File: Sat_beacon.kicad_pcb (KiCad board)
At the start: 4 copper layers, 123.9 x 79.5 mm, 126 parts, among them IC1 LMX2581ESQE_NOPB, IC2 LMX2581ESQE_NOPB, J1 Conn_01x05_Pin, J2 Conn_01x03_Pin, J4 SMA, J5 SMA, J6 Conn_01x04_Pin, Q1 BC817-40, Q2 BC817-40, Q3 BC817-40, Q4 BC817-40, SW1 B1407, SW2 SW_Omron_B3FS, SW3 SW_Omron_B3FS, SW4 SW_Omron_B3FS, SW5 SW_Omron_B3FS, U1 LD1117DT33, U2 LD1117DT33, U3 LD1117DT33, U4 1720BL15B0050002E, U5 1720BL15B0050002E, U7 STM32C031C6Tx, Y1 FT2MHUPM10.0-T1

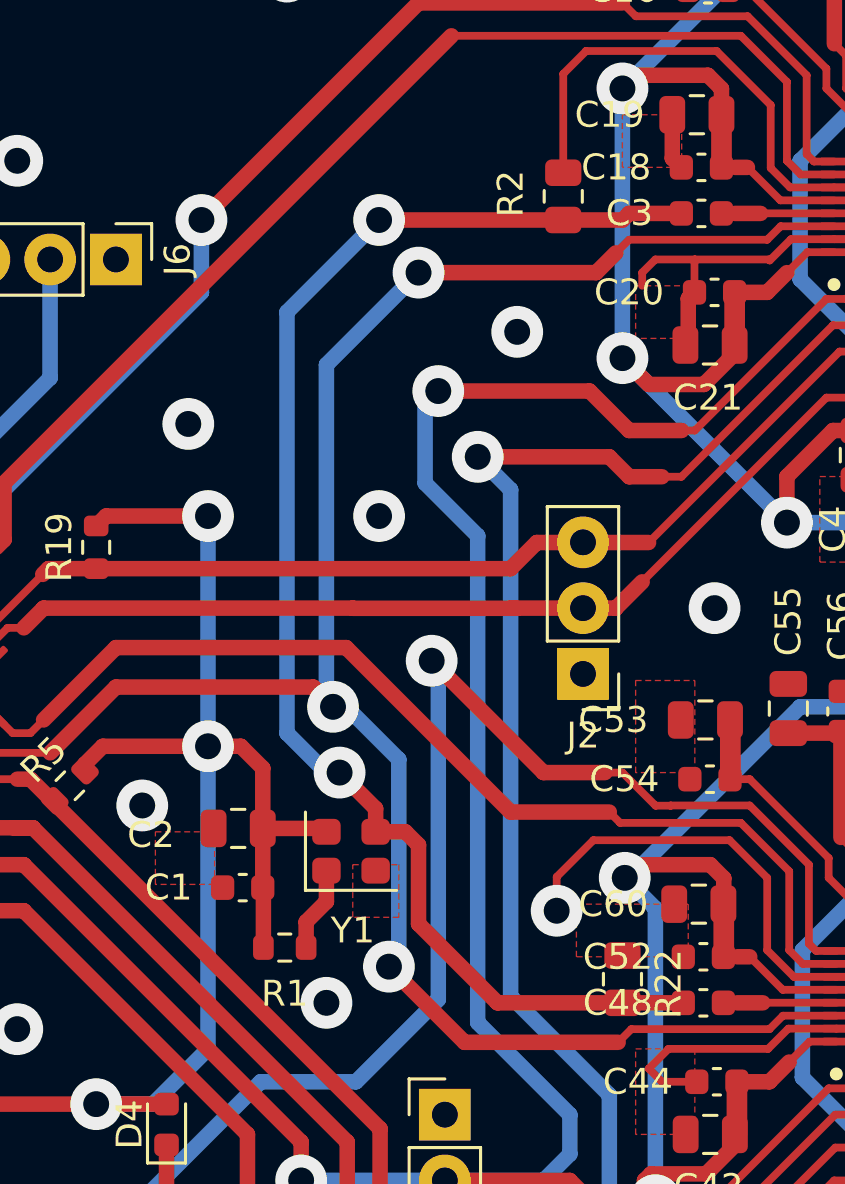
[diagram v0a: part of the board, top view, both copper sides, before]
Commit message: PCB improvements
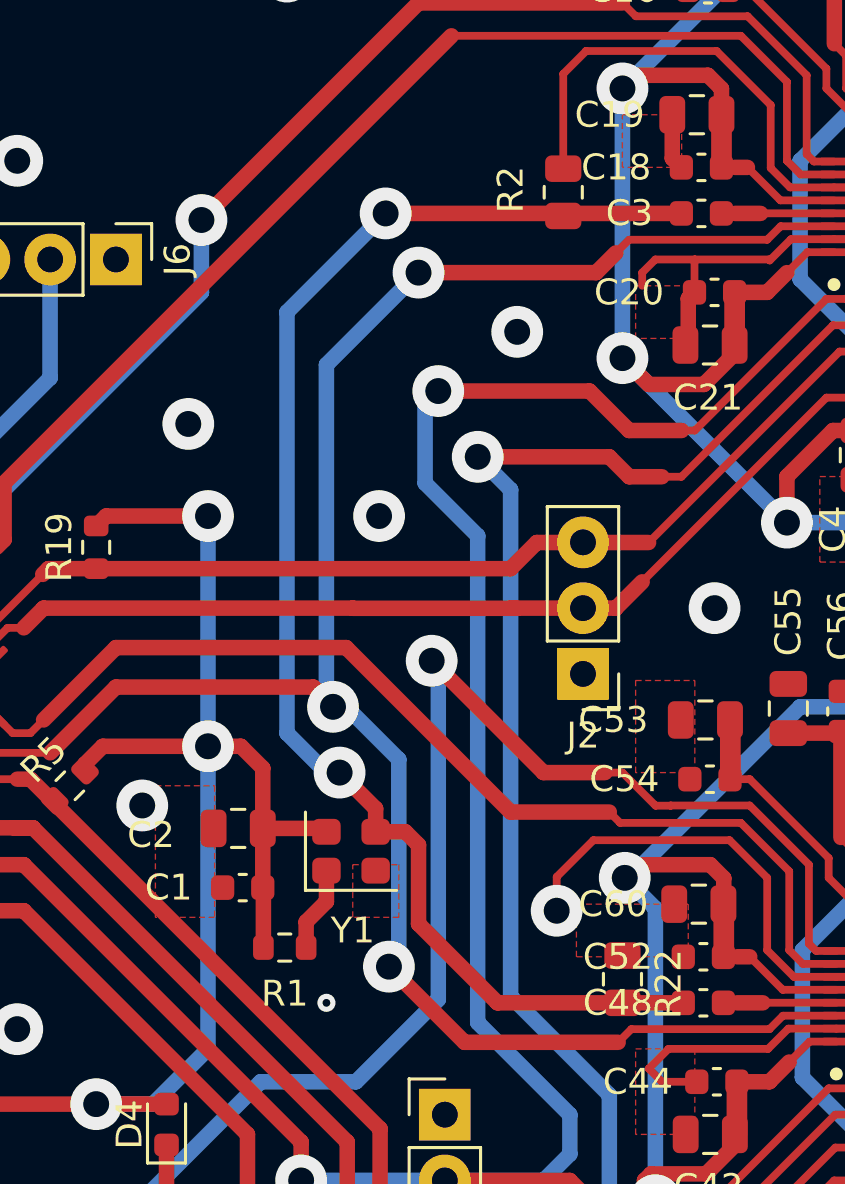
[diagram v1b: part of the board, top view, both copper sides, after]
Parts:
- moved R2 0.16 mm to (133.3, 75.7)
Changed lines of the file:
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@@
 	(footprint "Resistor_SMD:R_0805_2012Metric"
 		(layer "F.Cu")
-		(at 133.297317 75.857676 90)
+		(at 133.297317 75.700677 90)
 		(descr "Resistor SMD 0805 (2012 Metric), square (rectangular) end terminal, IPC-7351 nominal, (Body size source: IPC-SM-782 page 72, https://www.pcb-3d.com/wordpress/wp-content/uploads/ipc-sm-782a_amendment_1_and_2.pdf), generated with kicad-footprint-generator")
 		(tags "resistor")
@@
 	(via
 		(at 124.153317 106.996176)
-		(size 2)
-		(drill 1)
+		(size 0.7)
+		(drill 0.3)
 		(layers "F.Cu" "B.Cu")
 		(free yes)
@@
 	)
 	(segment
-		(start 135.837317 76.516177)
-		(end 135.583317 76.770176)
-		(width 0.6)
-		(layer "F.Cu")
-		(net 4)
-	)
-	(segment
 		(start 127.709317 100.900176)
 		(end 127.201318 100.392177)
@@
 	)
 	(segment
-		(start 135.583317 76.770176)
-		(end 133.297317 76.770176)
-		(width 0.6)
-		(layer "F.Cu")
-		(net 4)
-	)
-	(segment
 		(start 135.925593 106.996176)
 		(end 137.944592 106.996177)
@@
 	)
 	(segment
-		(start 133.297317 76.770176)
-		(end 126.185318 76.770176)
-		(width 0.6)
-		(layer "F.Cu")
-		(net 4)
-	)
-	(segment
 		(start 127.709317 103.948177)
 		(end 127.709317 100.900176)
@@
 	)
 	(segment
-		(start 135.837317 76.516177)
+		(start 126.439317 76.516177)
 		(end 137.856317 76.516177)
 		(width 0.6)
@@
 	)
 	(via
-		(at 126.185318 76.770176)
+		(at 126.439317 76.516177)
 		(size 2)
 		(drill 1)
@@
 	(segment
 		(start 124.153317 98.106177)
-		(end 122.629317 96.582177)
+		(end 124.661317 98.106176)
 		(width 0.6)
 		(layer "B.Cu")
@@
 	(segment
 		(start 122.629317 80.326177)
-		(end 126.185318 76.770176)
+		(end 122.629317 96.582177)
 		(width 0.6)
 		(layer "B.Cu")
@@
 	)
 	(segment
-		(start 122.629317 96.582177)
+		(start 126.439317 76.516177)
 		(end 122.629317 80.326177)
 		(width 0.6)
@@
 	)
 	(segment
-		(start 124.661317 98.106176)
+		(start 122.629317 96.582177)
 		(end 124.153317 98.106177)
 		(width 0.6)
@@
 		(name "$teardrop_padvia$")
 		(hatch none 0.1)
-		(priority 30002)
+		(priority 30003)
 		(attr
 			(teardrop
@@
 		(name "$teardrop_padvia$")
 		(hatch none 0.1)
-		(priority 30001)
+		(priority 30006)
 		(attr
 			(teardrop
@@
 		(name "$teardrop_padvia$")
 		(hatch none 0.1)
-		(priority 30005)
+		(priority 30001)
 		(attr
 			(teardrop
@@
 		(priority 1)
 		(connect_pads yes
-			(clearance 0.2)
+			(clearance 0.6)
 		)
 		(min_thickness 0.3)
@@
 		(polygon
 			(pts
-				(xy 117.549317 102.424177) (xy 117.549317 100.392177) (xy 119.835317 100.392177) (xy 119.835317 102.424177)
+				(xy 117.549317 103.694177) (xy 117.549317 98.614177) (xy 119.835317 98.614177) (xy 119.835317 103.694177)
 			)
 		)
@@
 		(name "$teardrop_padvia$")
 		(hatch none 0.1)
-		(priority 30006)
+		(priority 30005)
 		(attr
 			(teardrop
@@
 		(name "$teardrop_padvia$")
 		(hatch none 0.1)
-		(priority 30003)
+		(priority 30002)
 		(attr
 			(teardrop
@@
 		(name "$teardrop_padvia$")
 		(hatch none 0.1)
-		(priority 30015)
+		(priority 30012)
 		(attr
 			(teardrop
@@
 		(name "$teardrop_padvia$")
 		(hatch none 0.1)
-		(priority 30012)
+		(priority 30015)
 		(attr
 			(teardrop
